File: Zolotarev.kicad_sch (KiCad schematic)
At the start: 172 parts, among them J1 RF_IN, J2 RF_OUT, J3 Conn_02x05_Odd_Even, K1 G5LE-1, K10 G5LE-1, K11 G5LE-1, K12 G5LE-1, K13 G5LE-1, K14 G5LE-1, K2 G5LE-1, K3 G5LE-1, K4 G5LE-1, K5 G5LE-1, K6 G5LE-1, K7 G5LE-1, K8 G5LE-1, K9 G5LE-1

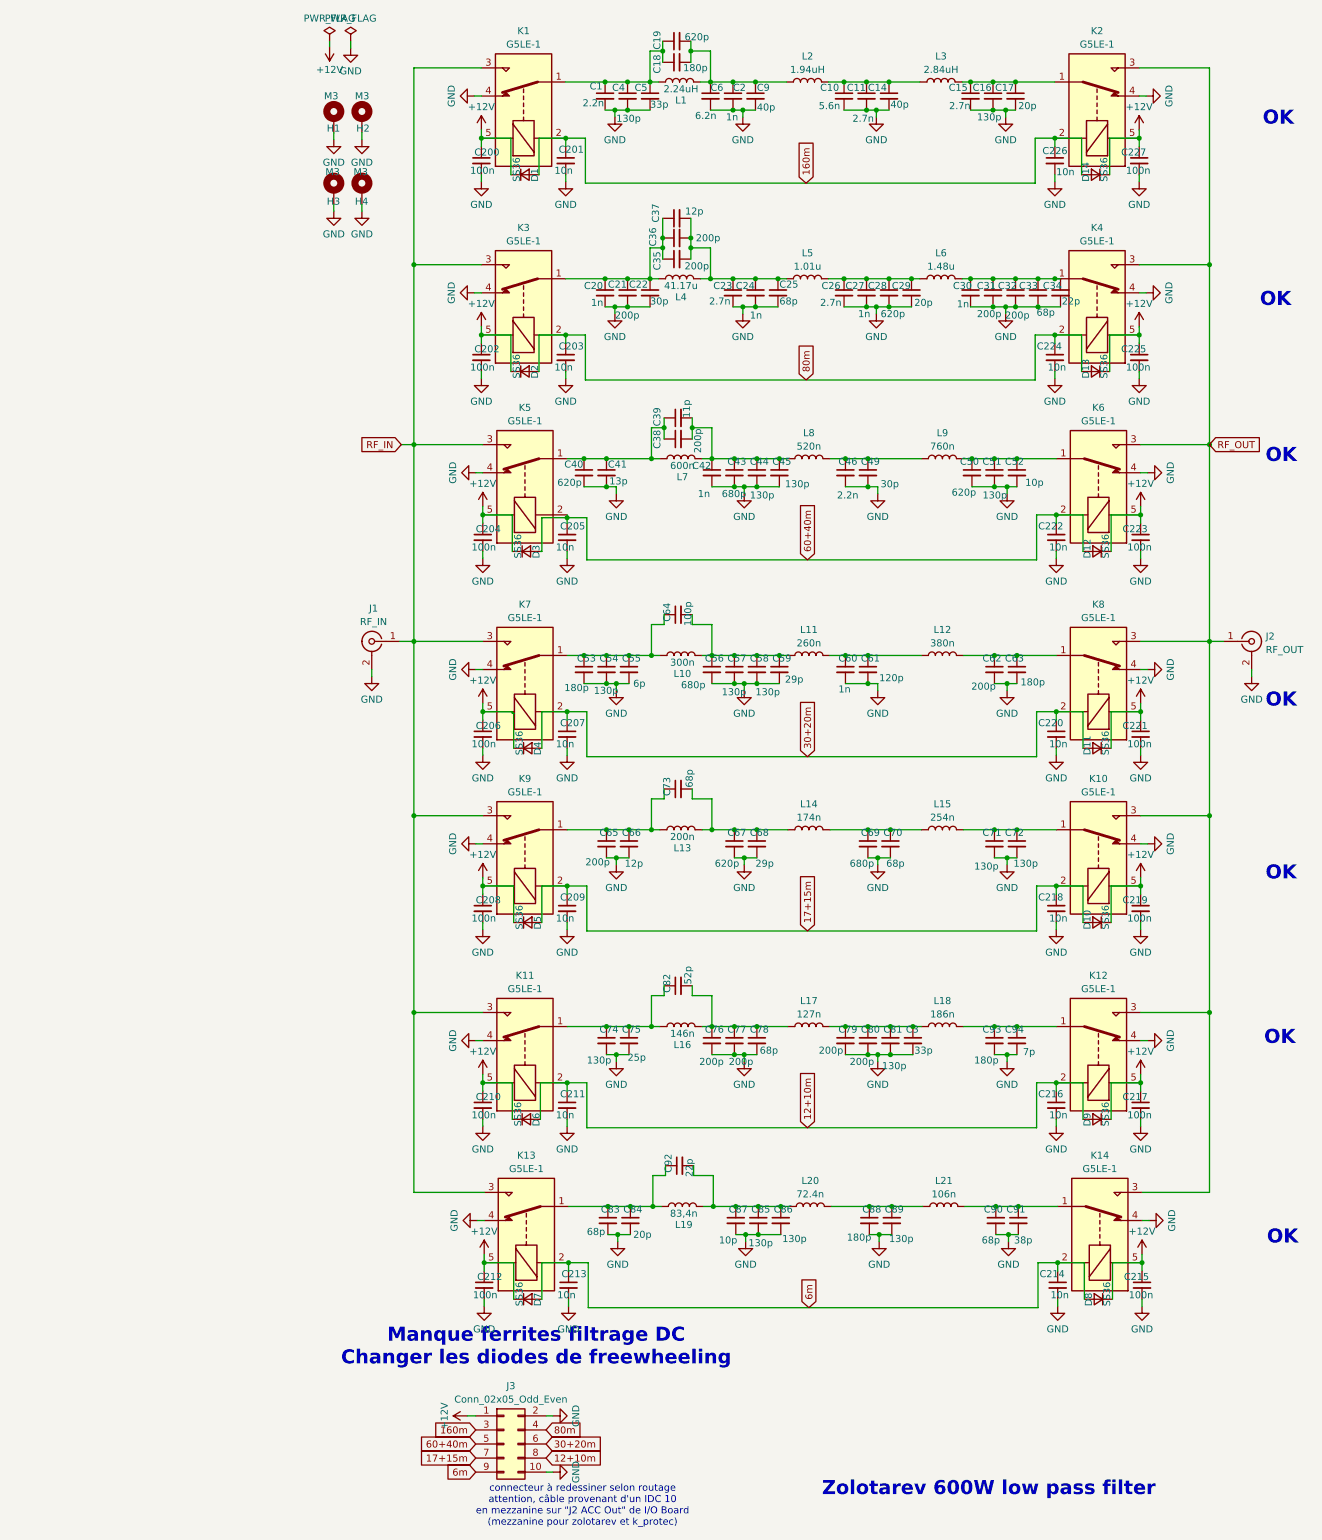
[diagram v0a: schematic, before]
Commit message: control connector and some ferrites later
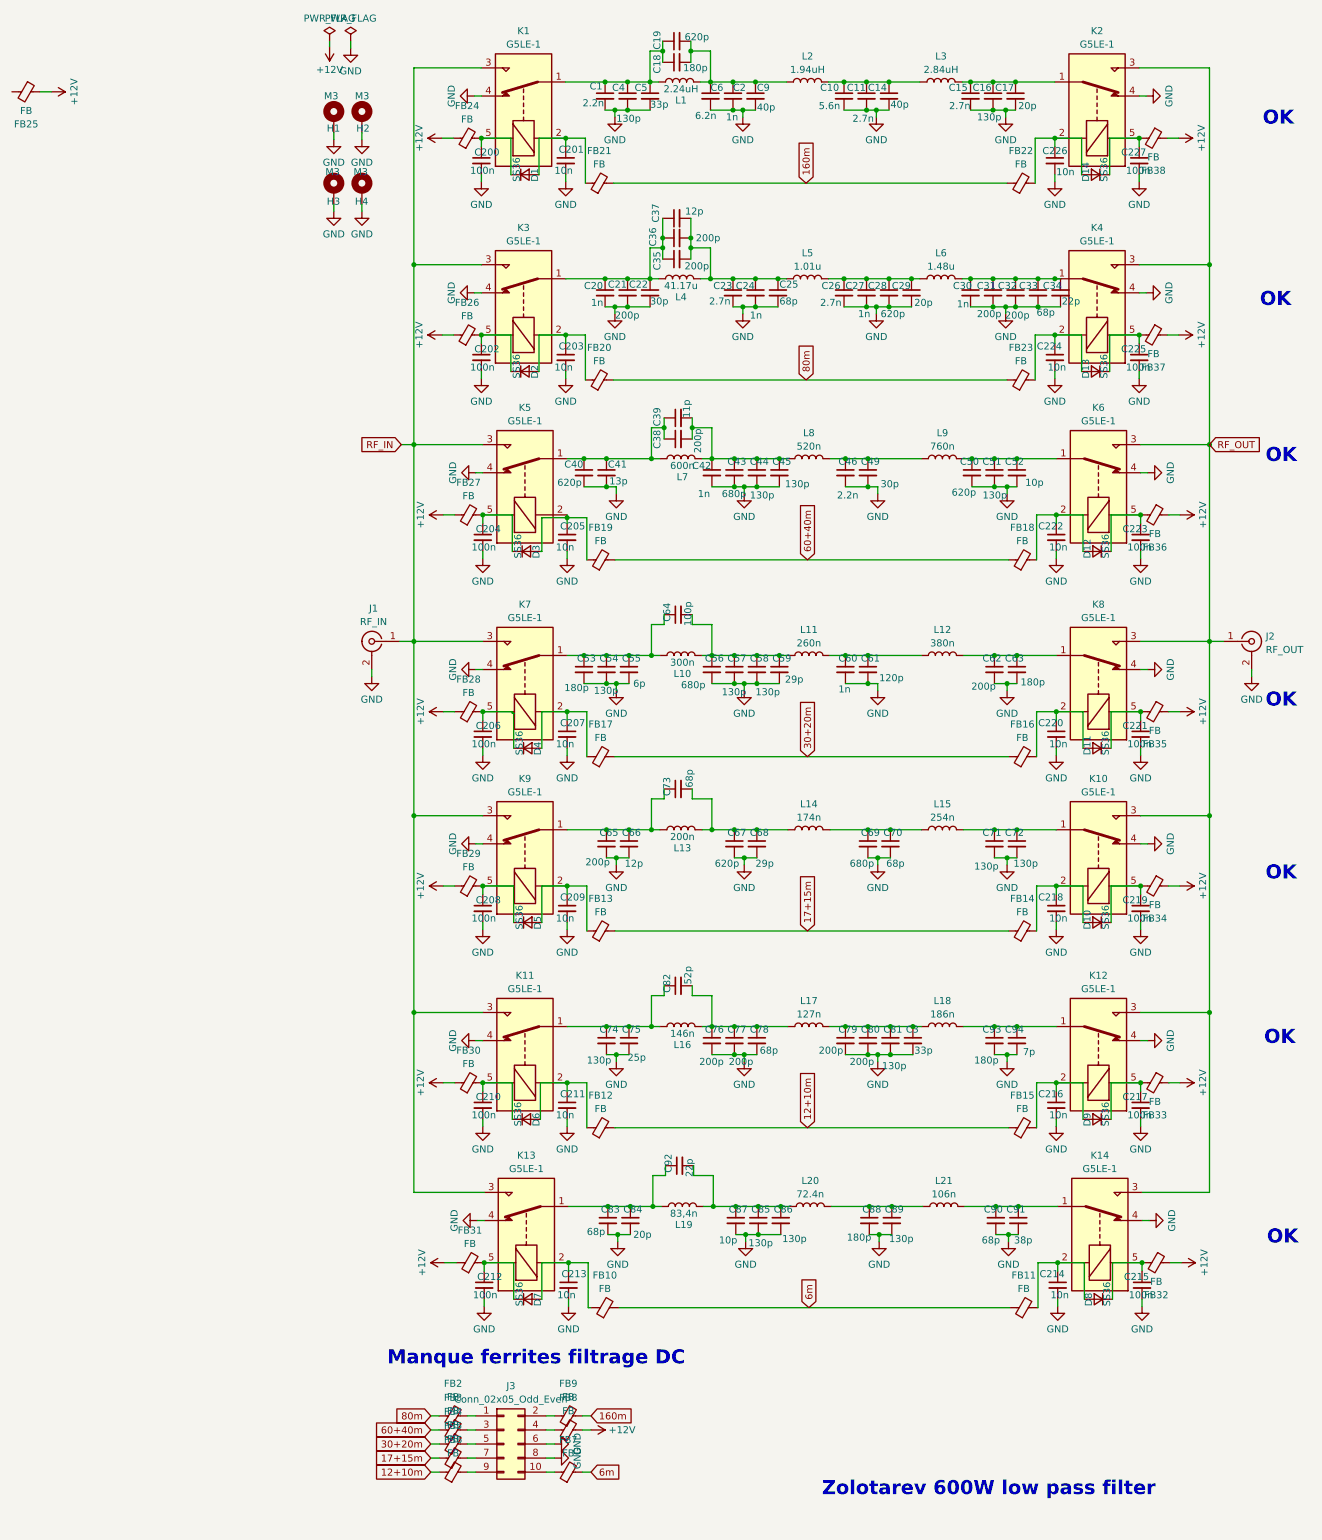
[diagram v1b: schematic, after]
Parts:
- added FB10, FB11, FB12, FB13, FB14, FB15, FB16, FB17, FB18, FB19, FB2, FB20, FB21, FB22, FB23, FB24, FB25, FB26, FB27, FB28, FB29, FB3, FB30, FB31, FB32, FB33, FB34, FB35, FB36, FB37, FB38, FB4, FB5, FB6, FB7, FB8, FB9: FB, Inductor_SMD:L_0805_2012Metric_Pad1.15x1.40mm_HandSolder, symbol Device:FerriteBead_Small
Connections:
- net +12V: now also FB24.1, FB25.1, FB26.1, FB27.1, FB28.1, FB29.1, FB30.1, FB31.1, FB32.1, FB33.1, FB34.1, FB35.1, FB36.1, FB37.1, FB38.1, FB8.2; no longer C200.1, C202.1, C204.1, C206.1, C208.1, C210.1, C212.1, C215.1, C217.1, C219.1, C221.1, C223.1, C225.1, C227.1, D1.1 (K), D10.1 (K), D11.1 (K), D12.1 (K), D13.1 (K), D14.1 (K), D2.1 (K), D3.1 (K), D4.1 (K), D5.1 (K), D6.1 (K), D7.1 (K), D8.1 (K), D9.1 (K), J3.1 (Pin_1), K1.5, K10.5, K11.5, K12.5, K13.5, K14.5, K2.5, K3.5, K4.5, K5.5, K6.5, K7.5, K8.5, K9.5
- net 12+10m: now also FB12.2, FB15.1, FB6.1; no longer C211.1, C216.1, D6.2 (A), D9.2 (A), J3.8 (Pin_8), K11.2, K12.2
- net 160m: now also FB21.2, FB22.1, FB9.2; no longer C201.1, C226.1, D1.2 (A), D14.2 (A), J3.3 (Pin_3), K1.2, K2.2
- net 17+15m: now also FB13.2, FB14.1, FB5.1; no longer C209.1, C218.1, D10.2 (A), D5.2 (A), J3.7 (Pin_7), K10.2, K9.2
- net 30+20m: now also FB16.1, FB17.2, FB4.1; no longer C207.1, C220.1, D11.2 (A), D4.2 (A), J3.6 (Pin_6), K7.2, K8.2
- net 60+40m: now also FB18.1, FB19.2, FB3.1; no longer C205.1, C222.1, D12.2 (A), D3.2 (A), J3.5 (Pin_5), K5.2, K6.2
- net 6m: now also FB10.2, FB11.1, FB7.2; no longer C213.1, C214.1, D7.2 (A), D8.2 (A), J3.9 (Pin_9), K13.2, K14.2
- net 80m: now also FB2.1, FB20.2, FB23.1; no longer C203.1, C224.1, D13.2 (A), D2.2 (A), J3.4 (Pin_4), K3.2, K4.2
- net GND: now also J3.6 (Pin_6), J3.8 (Pin_8); no longer J3.10 (Pin_10), J3.2 (Pin_2)
- new net: FB2.2, J3.1 (Pin_1)
- new net: C205.1, D3.2 (A), FB19.1, K5.2
- new net: C225.1, D13.1 (K), FB37.2, K4.5
- new net: C224.1, D13.2 (A), FB23.2, K4.2
- new net: FB8.1, J3.4 (Pin_4)
- new net: FB3.2, J3.3 (Pin_3)
- new net: C202.1, D2.1 (K), FB26.2, K3.5
- new net: C203.1, D2.2 (A), FB20.1, K3.2
- new net: FB6.2, J3.9 (Pin_9)
- new net: C220.1, D11.2 (A), FB16.2, K8.2
- new net: C207.1, D4.2 (A), FB17.1, K7.2
- new net: C214.1, D8.2 (A), FB11.2, K14.2
- new net: C204.1, D3.1 (K), FB27.2, K5.5
- new net: C201.1, D1.2 (A), FB21.1, K1.2
- new net: C216.1, D9.2 (A), FB15.2, K12.2
- new net: C213.1, D7.2 (A), FB10.1, K13.2
- new net: C200.1, D1.1 (K), FB24.2, K1.5
- new net: C206.1, D4.1 (K), FB28.2, K7.5
- new net: FB5.2, J3.7 (Pin_7)
- new net: C209.1, D5.2 (A), FB13.1, K9.2
- new net: FB7.1, J3.10 (Pin_10)
- new net: C226.1, D14.2 (A), FB22.2, K2.2
- new net: C218.1, D10.2 (A), FB14.2, K10.2
- new net: C223.1, D12.1 (K), FB36.2, K6.5
- new net: C221.1, D11.1 (K), FB35.2, K8.5
- new net: C222.1, D12.2 (A), FB18.2, K6.2
- new net: C215.1, D8.1 (K), FB32.2, K14.5
- new net: C212.1, D7.1 (K), FB31.2, K13.5
- new net: C227.1, D14.1 (K), FB38.2, K2.5
- new net: C210.1, D6.1 (K), FB30.2, K11.5
- new net: C219.1, D10.1 (K), FB34.2, K10.5
- new net: C217.1, D9.1 (K), FB33.2, K12.5
- new net: FB9.1, J3.2 (Pin_2)
- new net: FB4.2, J3.5 (Pin_5)
- new net: C208.1, D5.1 (K), FB29.2, K9.5
- new net: C211.1, D6.2 (A), FB12.1, K11.2
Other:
- note added: "Manque ferrites filtrage DC"
- note removed: "Manque ferrites filtrage DC Changer les diodes de freewheeling"
- note removed: "connecteur à redessiner selon routage attention, câble provenant d'un IDC 10 en mezzanine sur "J2 ACC Out" de I/O Board (mezzanine pour zolotarev et k_protec)"
